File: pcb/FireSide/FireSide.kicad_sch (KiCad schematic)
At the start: 27 parts, among them J0 SDIOModule, J1 D4184_PIN_A, J10 5V_01x02_JST, J11 5V_01x02_JST, J12 Status_01x02_JST, J2 D4184_PIN_B, J3 D4184_PIN_C, J4 A0_01x02_JST, J5 A1_01x02_JST, J6 A2_01x02_JST, J60 XT60-Male, J7 A3_01x02_JST, J8 A4_01x02_JST, J9 A5_01x02_JST, Q1 MMBT2222A, U1 AMS1117-5.0, U3 RYLR998

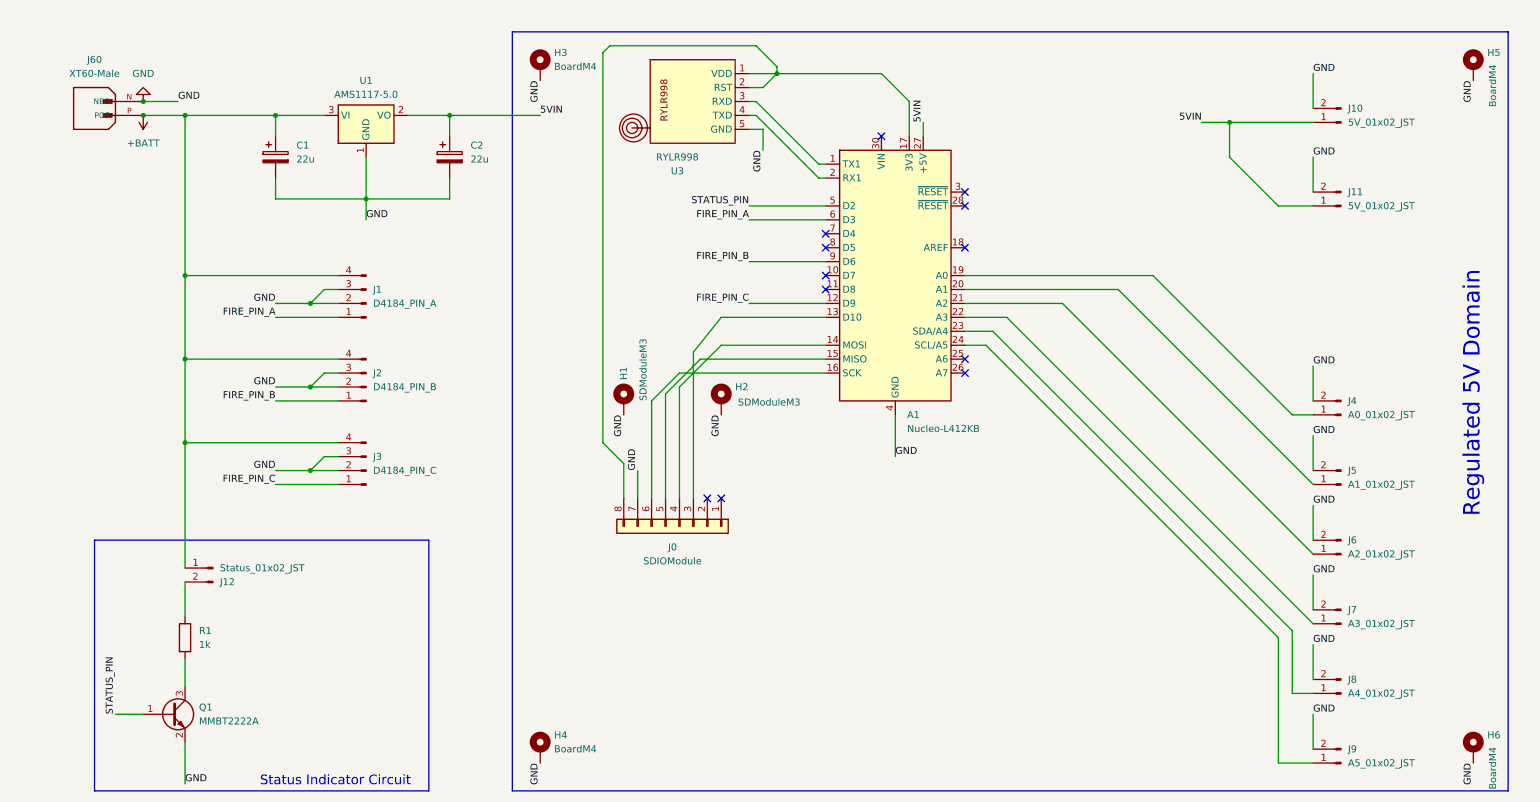
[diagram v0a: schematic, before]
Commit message: [FS] PCB Updated to v1.1.6
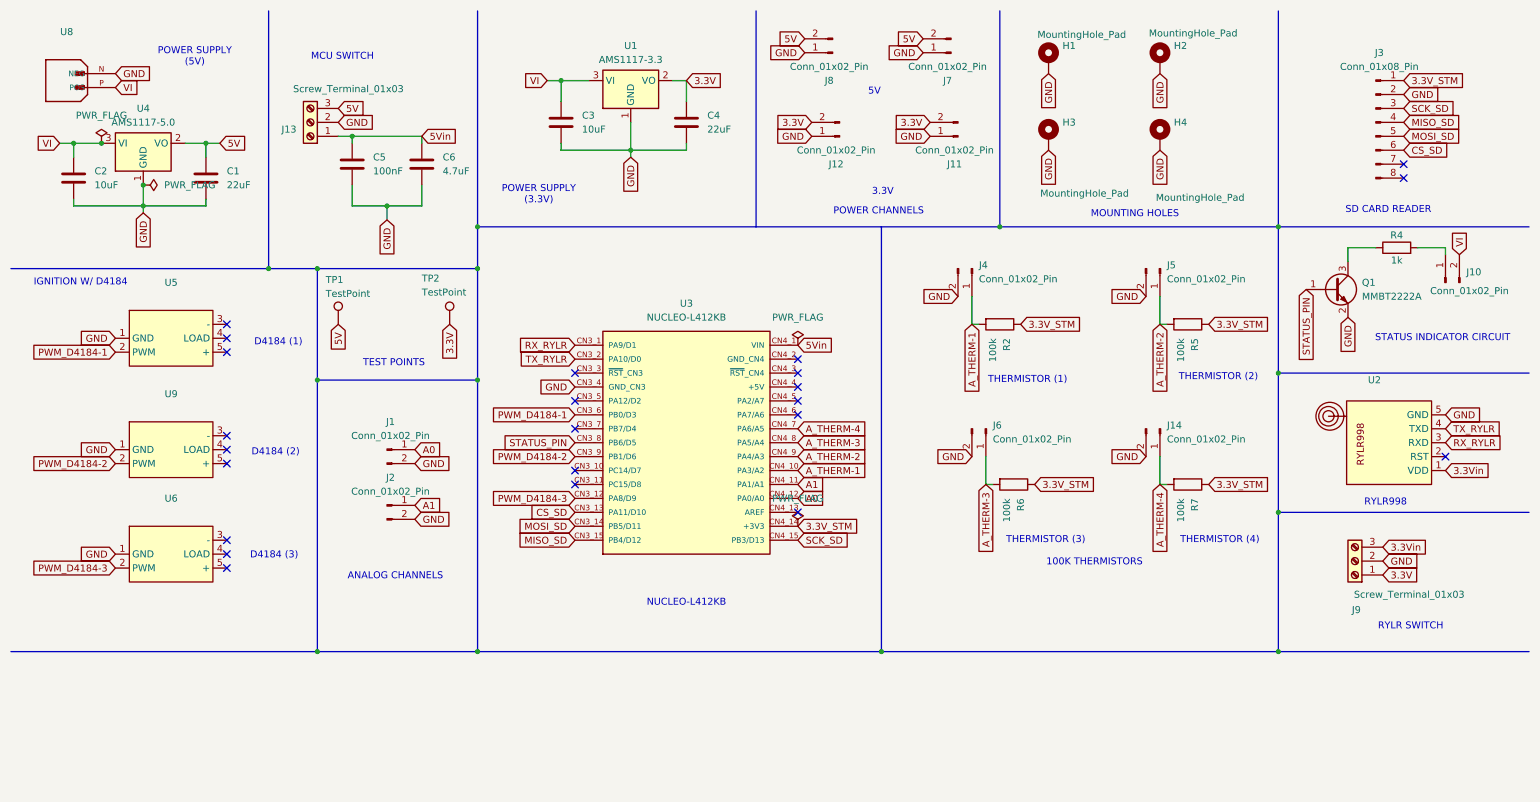
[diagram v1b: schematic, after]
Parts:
- removed A1: Nucleo-L412KB, Module:Arduino_Nano, symbol MCU_Module:Arduino_Nano_Every
- removed C1, C2: 22u, Capacitor_THT:CP_Radial_D5.0mm_P2.50mm, symbol Device:C_Polarized
- removed H5, H6: BoardM4, MountingHole:MountingHole_4.3mm_M4_ISO7380_Pad_TopBottom, symbol Mechanical:MountingHole_Pad
- removed J0: SDIOModule, Connector_Molex:Molex_Nano-Fit_105309-xx08_1x08_P2.50mm_Vertical, symbol Connector_Generic:Conn_01x08
- removed J1: D4184_PIN_A, Connector_JST:JST_XH_B4B-XH-A_1x04_P2.50mm_Vertical, symbol Connector:Conn_01x04_Pin
- removed J2: D4184_PIN_B, Connector_JST:JST_XH_B4B-XH-A_1x04_P2.50mm_Vertical, symbol Connector:Conn_01x04_Pin
- removed J3: D4184_PIN_C, Connector_JST:JST_XH_B4B-XH-A_1x04_P2.50mm_Vertical, symbol Connector:Conn_01x04_Pin
- removed J60: XT60-Male, XT60-M:AMASS_XT60-M, symbol XT60-M:XT60-M
- removed J9: A5_01x02_JST, Connector_JST:JST_XH_B2B-XH-A_1x02_P2.50mm_Vertical, symbol Connector:Conn_01x02_Pin
- removed R1: 1k, Resistor_SMD:R_0805_2012Metric_Pad1.20x1.40mm_HandSolder, symbol Device:R
- removed U1: AMS1117-5.0, Package_TO_SOT_SMD:SOT-223-3_TabPin2, symbol Regulator_Linear:AMS1117-5.0
- removed U3: RYLR998, RYLR998:RYLR998, symbol RYLR998:RYLR998
- added C1, C4: 22uF, Capacitor_SMD:C_0805_2012Metric, symbol Device:C
- added C2, C3: 10uF, Capacitor_SMD:C_0805_2012Metric, symbol Device:C
- added C5: 100nF, Capacitor_SMD:C_0805_2012Metric, symbol Device:C
- added C6: 4.7uF, Capacitor_SMD:C_0805_2012Metric, symbol Device:C
- added J1, J14, J2: Conn_01x02_Pin, Connector_JST:JST_XH_B2B-XH-A_1x02_P2.50mm_Vertical, symbol Connector:Conn_01x02_Pin
- added J13, J9: Screw_Terminal_01x03, TerminalBlock:TerminalBlock_bornier-3_P5.08mm, symbol Connector:Screw_Terminal_01x03
- added J3: Conn_01x08_Pin, Connector_PinHeader_2.54mm:PinHeader_1x08_P2.54mm_Vertical, symbol Connector:Conn_01x08_Pin
- added R2, R5, R6, R7: 100k, Resistor_THT:R_Axial_DIN0204_L3.6mm_D1.6mm_P5.08mm_Horizontal, symbol Device:R
- added R4: 1k, Resistor_SMD:R_0805_2012Metric, symbol Device:R
- added TP1, TP2: TestPoint, TestPoint:TestPoint_Loop_D2.60mm_Drill1.6mm_Beaded, symbol Connector:TestPoint
- added U1: AMS1117-3.3, Package_TO_SOT_SMD:SOT-223-3_TabPin2, symbol Regulator_Linear:AMS1117-3.3
- added U2: ~, FireSide Footprint:RYLR998, symbol FireSide symbol:RYLR998
- added U3: NUCLEO-L412KB, FireSide Footprint:NUCLEO-L412KB, symbol FireSide symbol:NUCLEO-L412KB
- added U4: AMS1117-5.0, Package_TO_SOT_SMD:SOT-223-3_TabPin2, symbol Regulator_Linear:AMS1117-5.0
- added U5, U6, U9: ~, FireSide Footprint:D4184, symbol FireSide symbol:D4184
- added U8: ~, FireSide Footprint:XT60-M, symbol FireSide symbol:XT60-M
- H1, H2: value SDModuleM3 -> MountingHole_Pad; footprint MountingHole:MountingHole_3.2mm_M3_ISO7380_Pad_TopBottom -> MountingHole:MountingHole_4.3mm_M4_DIN965_Pad
- H3, H4: value BoardM4 -> MountingHole_Pad; footprint MountingHole:MountingHole_4.3mm_M4_ISO7380_Pad_TopBottom -> MountingHole:MountingHole_4.3mm_M4_DIN965_Pad
- J10, J11: value 5V_01x02_JST -> Conn_01x02_Pin
- J12: value Status_01x02_JST -> Conn_01x02_Pin
- J4: value A0_01x02_JST -> Conn_01x02_Pin
- J5: value A1_01x02_JST -> Conn_01x02_Pin
- J6: value A2_01x02_JST -> Conn_01x02_Pin
- J7: value A3_01x02_JST -> Conn_01x02_Pin
- J8: value A4_01x02_JST -> Conn_01x02_Pin
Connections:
- net +BATT is gone; now on net GND: J12.1 (Pin_1)
- net GND: now also J11.1 (Pin_1), J7.1 (Pin_1), J8.1 (Pin_1), C1.2, C2.2, C3.2, C4.2, C5.2, C6.2, J1.2 (Pin_2), J13.2 (Pin_2), J14.2 (Pin_2), J2.2 (Pin_2), J3.2 (Pin_2), J9.2 (Pin_2), U1.1 (GND), U2.5 (GND), U3.CN3_4 (GND_CN3), U4.1 (GND), U5.1 (GND), U6.1 (GND), U8.N (NEG), U9.1 (GND); no longer J10.2 (Pin_2), J11.2 (Pin_2), J7.2 (Pin_2), J8.2 (Pin_2)
- net STATUS_PIN: now also U3.CN3_8 (PB6/D5)
- net A_THERM-2: now reaches J5.1 (Pin_1)
- net A_THERM-2: now also R5.2, U3.CN4_9 (PA4/A3)
- net 3.3V: now reaches J12.2 (Pin_2)
- net 3.3V: now also J11.2 (Pin_2), C4.1, J9.1 (Pin_1), TP2.1, U1.2 (VO)
- net at Q1.3 (C): now also R4.1
- net A_THERM-1: now reaches J4.1 (Pin_1)
- net A_THERM-1: now also R2.2, U3.CN4_10 (PA3/A2)
- net A_THERM-3: now reaches J6.1 (Pin_1)
- net A_THERM-3: now also R6.2, U3.CN4_8 (PA5/A4)
- net 5VIN: no longer names the net of J10.1 (Pin_1)
- net 5VIN: now also R4.2; no longer J11.1 (Pin_1)
- new net 3.3V_STM: J3.1 (Pin_1), R2.1, R5.1, R6.1, R7.1, U3.CN4_14 (+3V3)
- new net 3.3Vin: J9.3 (Pin_3), U2.1 (VDD)
- new net 5V: C1.1, J13.3 (Pin_3), J7.2 (Pin_2), J8.2 (Pin_2), TP1.1, U4.2 (VO)
- new net 5Vin: C5.1, C6.1, J13.1 (Pin_1), U3.CN4_1 (VIN)
- new net A0: J1.1 (Pin_1), U3.CN4_12 (PA0/A0)
- new net A1: J2.1 (Pin_1), U3.CN4_11 (PA1/A1)
- new net A_THERM-4: J14.1 (Pin_1), R7.2, U3.CN4_7 (PA6/A5)
- new net CS_SD: J3.6 (Pin_6), U3.CN3_13 (PA11/D10)
- new net MISO_SD: J3.4 (Pin_4), U3.CN3_15 (PB4/D12)
- new net MOSI_SD: J3.5 (Pin_5), U3.CN3_14 (PB5/D11)
- new net PWM_D4184-1: U3.CN3_6 (PB0/D3), U5.2 (PWM)
- new net PWM_D4184-2: U3.CN3_9 (PB1/D6), U9.2 (PWM)
- new net PWM_D4184-3: U3.CN3_12 (PA8/D9), U6.2 (PWM)
- new net RX_RYLR: U2.3 (RXD), U3.CN3_1 (PA9/D1)
- new net SCK_SD: J3.3 (Pin_3), U3.CN4_15 (PB3/D13)
- new net TX_RYLR: U2.4 (TXD), U3.CN3_2 (PA10/D0)
- new net VI: C2.1, C3.1, J10.2 (Pin_2), U1.3 (VI), U4.3 (VI), U8.P (POS)
- no-connect marks 12 -> 23
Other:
- note added: "100K THERMISTORS"
- note added: "3.3V"
- note added: "5V"
- note added: "ANALOG CHANNELS"
- note added: "D4184 (1)"
- note added: "D4184 (2)"
- note added: "D4184 (3)"
- note added: "IGNITION W/ D4184"
- note added: "MCU SWITCH"
- note added: "MOUNTING HOLES"
- note added: "NUCLEO-L412KB"
- note added: "POWER CHANNELS"
- note added: "POWER SUPPLY (3.3V)"
- note added: "POWER SUPPLY (5V)"
- note added: "RYLR SWITCH"
- note added: "RYLR998"
- note added: "SD CARD READER"
- note added: "STATUS INDICATOR CIRCUIT"
- note added: "TEST POINTS"
- note added: "THERMISTOR (1)"
- note added: "THERMISTOR (2)"
- note added: "THERMISTOR (3)"
- note added: "THERMISTOR (4)"
- note removed: "Regulated 5V Domain"
- note removed: "Status Indicator Circuit"
- title: FireSide -> FireSide v2.0
